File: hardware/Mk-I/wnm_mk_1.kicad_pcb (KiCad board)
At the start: 2 copper layers, 96.5 x 67.1 mm, 126 parts, among them CON1 10118194-0001LF, SW1 EVQ-Q2S02W, SW10 EVQ-Q2S02W, SW11 EVQ-Q2S02W, SW12 EVQ-Q2S02W, SW13 EVQ-Q2S02W, SW14 EVQ-Q2S02W, SW15 EVQ-Q2S02W, SW16 EVQ-Q2S02W, SW18 EVQ-Q2S02W, SW19 EVQ-Q2S02W, SW2 EVQ-Q2S02W, SW20 EVQ-Q2S02W, SW21 EVQ-Q2S02W, SW22 EVQ-Q2S02W, SW3 EVQ-Q2S02W, SW4 EVQ-Q2S02W, SW5 EVQ-Q2S02W, SW6 EVQ-Q2S02W, SW7 EVQ-Q2S02W, SW8 EVQ-Q2S02W, SW9 EVQ-Q2S02W, U1 AP7313-18SRG-7, U10 STM32_SWD_Connector, U2 MCP73831T-2ACI/OT, U3 BD33IA5MEFJ-ME2, U4 STM32F427VIT6, U5 SGTL5000XNAA3R2, U6 EC12D1524403, U7 EC12D1524403, U8 47219-2001, U9 SSD1306, X1 ABM3B-8.000MHZ-B2-T

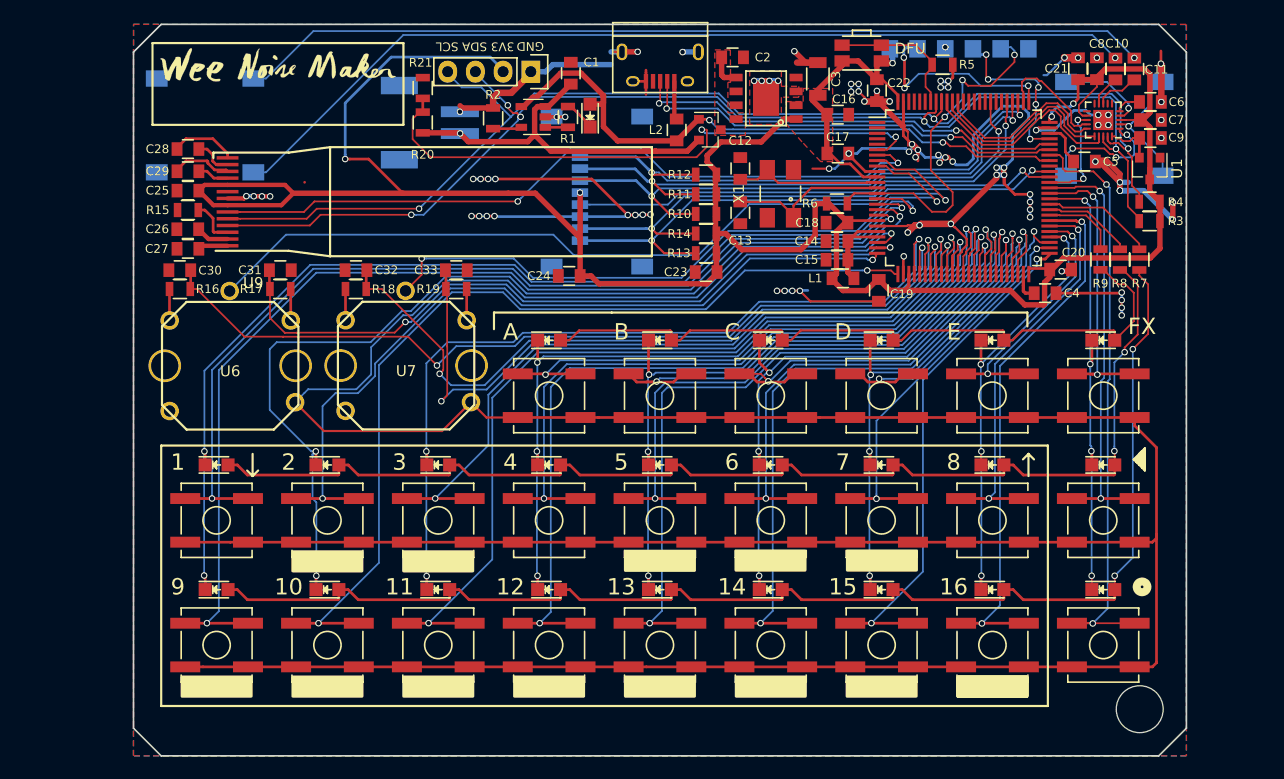
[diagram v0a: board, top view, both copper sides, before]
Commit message: HW: Major change of layout...
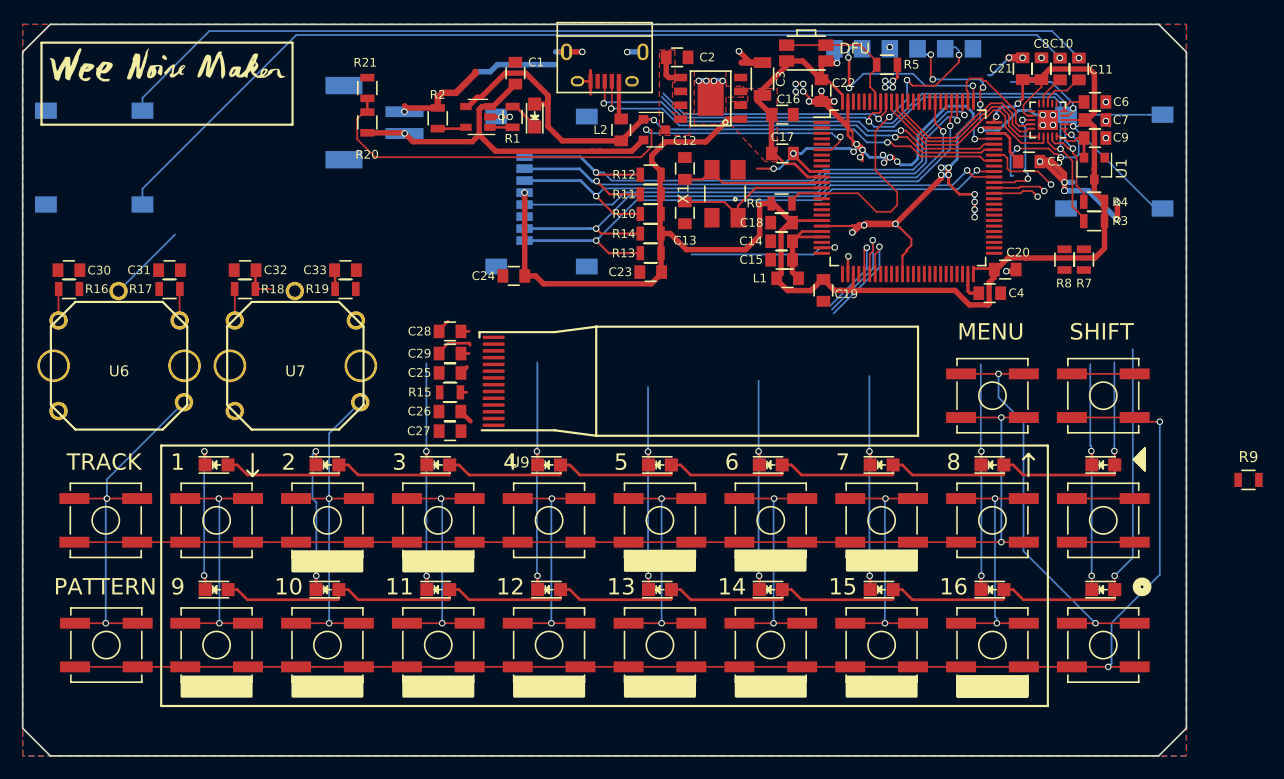
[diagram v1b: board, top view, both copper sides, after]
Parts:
- removed D20, D21, D22, D23, D24: 150060GS75000, LEDs:LED_0805
- removed D25: 150060RS75000, LEDs:LED_0805
- removed REF**: MountingHole_4.3mm_M4, Mounting_Holes:MountingHole_4.3mm_M4
- removed SW18, SW19: EVQ-Q2S02W, Buttons_Switches_SMD:SW_SPST_B3SL-1002P
- removed ext1: CONN_01X04, Socket_Strips:Socket_Strip_Straight_1x04
- R9: value 330 -> 10K
- moved SW21 72.0 mm to (77.5, 123.2)
- moved SW20 65.1 mm to (77.5, 134.6)
- moved U9 29.4 mm to (111.8, 114.8)
- moved C25 29.3 mm to (109.0, 109.7)
- moved C27 29.3 mm to (109.0, 115.0)
- moved C28 29.3 mm to (109.0, 105.9)
- moved R15 29.3 mm to (109.0, 111.5)
- moved C29 29.3 mm to (109.0, 107.9)
- moved C26 29.3 mm to (109.0, 113.2)
- moved R9 24.3 mm to (182.2, 119.5), turned to 0 degrees
- moved LINE_IN1 10.6 mm to (72.0, 94.2)
- moved U6 10.2 mm to (78.7, 109.0)
- moved C30 10.2 mm to (74.1, 100.3)
- moved C31 10.2 mm to (83.3, 100.3)
- moved C32 10.2 mm to (90.2, 100.3)
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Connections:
- Play1 pad 1: Play -> 3V3
- Play1 pad 2: WAKEUP -> Play_WKUP
- Play2 pad 1: FX -> BUTTON_COL11
- Play2 pad 2: WAKEUP -> BUTTON_ROW2
- R9 pad 1: ROW3 -> GND
- R9 pad 2: Net-(D20-Pad2) -> Play_WKUP
- SW1 pad 1: B1 -> BUTTON_COL2
- SW1 pad 2: WAKEUP -> BUTTON_ROW1
- SW10 pad 1: B10 -> BUTTON_COL3
- SW10 pad 2: WAKEUP -> BUTTON_ROW2
- SW11 pad 1: B11 -> BUTTON_COL4
- SW11 pad 2: WAKEUP -> BUTTON_ROW2
- SW12 pad 1: B12 -> BUTTON_COL5
- SW12 pad 2: WAKEUP -> BUTTON_ROW2
- SW13 pad 1: B13 -> BUTTON_COL6
- SW13 pad 2: WAKEUP -> BUTTON_ROW2
- SW14 pad 1: B14 -> BUTTON_COL7
- SW14 pad 2: WAKEUP -> BUTTON_ROW2
- SW15 pad 1: B15 -> BUTTON_COL8
- SW15 pad 2: WAKEUP -> BUTTON_ROW2
- SW16 pad 1: B16 -> BUTTON_COL9
- SW16 pad 2: WAKEUP -> BUTTON_ROW2
- SW2 pad 1: B2 -> BUTTON_COL3
- SW2 pad 2: WAKEUP -> BUTTON_ROW1
- SW20 pad 1: BC -> BUTTON_COL1
- SW20 pad 2: WAKEUP -> BUTTON_ROW2
- SW21 pad 1: BD -> BUTTON_COL1
- SW21 pad 2: WAKEUP -> BUTTON_ROW1
- SW22 pad 1: BE -> BUTTON_COL10
- SW22 pad 2: WAKEUP -> BUTTON_ROW1
- SW3 pad 1: B3 -> BUTTON_COL4
- SW3 pad 2: WAKEUP -> BUTTON_ROW1
- SW4 pad 1: B4 -> BUTTON_COL5
- SW4 pad 2: WAKEUP -> BUTTON_ROW1
- SW5 pad 1: B5 -> BUTTON_COL6
- SW5 pad 2: WAKEUP -> BUTTON_ROW1
- SW6 pad 1: B6 -> BUTTON_COL7
- SW6 pad 2: WAKEUP -> BUTTON_ROW1
- SW7 pad 1: B7 -> BUTTON_COL8
- SW7 pad 2: WAKEUP -> BUTTON_ROW1
- SW8 pad 1: B8 -> BUTTON_COL9
- SW8 pad 2: WAKEUP -> BUTTON_ROW1
- SW9 pad 1: B9 -> BUTTON_COL2
- SW9 pad 2: WAKEUP -> BUTTON_ROW2
- U4 pad 16: B1 -> Net-(U4-Pad16)
- U4 pad 18: B9 -> Net-(U4-Pad18)
- U4 pad 23: WAKEUP -> PLAY_WAKEUP
- U4 pad 25: B2 -> Net-(U4-Pad25)
- U4 pad 33: B3 -> Net-(U4-Pad33)
- U4 pad 34: B11 -> Net-(U4-Pad34)
- U4 pad 36: BA -> Net-(U4-Pad36)
- U4 pad 38: B4 -> Net-(U4-Pad38)
- U4 pad 39: B12 -> Net-(U4-Pad39)
- U4 pad 41: BB -> Net-(U4-Pad41)
- U4 pad 42: B5 -> Net-(U4-Pad42)
- U4 pad 43: B13 -> Net-(U4-Pad43)
- U4 pad 45: BC -> Net-(U4-Pad45)
- U4 pad 46: B6 -> Net-(U4-Pad46)
- U4 pad 47: B14 -> Net-(U4-Pad47)
- U4 pad 51: B15 -> Net-(U4-Pad51)
- U4 pad 52: B7 -> Net-(U4-Pad52)
- U4 pad 53: BD -> Net-(U4-Pad53)
- U4 pad 55: BE -> Net-(U4-Pad55)
- U4 pad 56: B8 -> Net-(U4-Pad56)
- U4 pad 57: B16 -> Net-(U4-Pad57)
- U4 pad 58: ROW3 -> Net-(U4-Pad58)
- U4 pad 62: FX -> Net-(U4-Pad62)
- U4 pad 63: Play -> Net-(U4-Pad63)
- U6 pad 4: WAKEUP -> BUTTON_COL1
- U6 pad 5: ENC_1_SW -> BUTTON_ROW3
- U7 pad 4: WAKEUP -> BUTTON_COL3
- U7 pad 5: ENC_2_SW -> BUTTON_ROW3
- Write1 pad 1: Write -> BUTTON_COL10
- Write1 pad 2: WAKEUP -> BUTTON_ROW2
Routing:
- net WAKEUP: track 348.3 -> 0.00 mm, vias 1 -> 0
- net BUTTON_ROW2: track 0.00 -> 129.8 mm, vias 0 -> 2
- net BUTTON_ROW1: track 0.00 -> 104.2 mm, vias 0 -> 2
- net B9: track 101.4 -> 0.00 mm, vias 2 -> 0
- net B1: track 93.1 -> 0.00 mm, vias 2 -> 0
- net B10: track 86.3 -> 0.00 mm, vias 2 -> 0
- net COL1: track 98.4 -> 14.0 mm, vias 3 -> 2
- net B11: track 82.3 -> 0.00 mm, vias 2 -> 0
- net B12: track 80.9 -> 0.00 mm, vias 2 -> 0
- net ENC_1_SW: track 78.9 -> 0.00 mm, vias 1 -> 0
- net COL2: track 92.3 -> 14.2 mm, vias 3 -> 2
- net B2: track 75.5 -> 0.00 mm, vias 2 -> 0
- net B3: track 72.2 -> 0.00 mm, vias 2 -> 0
- net B13: track 70.8 -> 0.00 mm, vias 2 -> 0
- net ENC_1_A: track 79.9 -> 9.21 mm, vias 2 -> 1
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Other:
- board size 96.5 x 67.1 mm -> 106.7 x 67.1 mm
- board text added: "MENU"
- board text added: "PATTERN"
- board text added: "SHIFT"
- board text added: "TRACK"
- board text removed: "3V3"
- board text removed: "A"
- board text removed: "B"
- board text removed: "C"
- board text removed: "D"
- board text removed: "E"
- board text removed: "FX"
- board text removed: "SCL"
- board text removed: "SDA"
